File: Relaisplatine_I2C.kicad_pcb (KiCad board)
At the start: 2 copper layers, 85.1 x 107.3 mm, 35 parts, among them J1 J, J1.1 G1-J, J1.2 G1-K, J1001 Conn_01x08, J2 K, J2.1 G2-J, J2.2 G2-K, J3.1 G3-J, J3.2 G3-K, J4.1 G4-J, J4.2 G4-K, J5.1 G5-J, J5.2 G5-K, J6.1 G6-J, J6.2 G6-K, J7.1 G7-J, J7.2 G7-K, J8.1 G8-J, J8.2 G8-K, U1 ULN2803A, U2 PCF8574

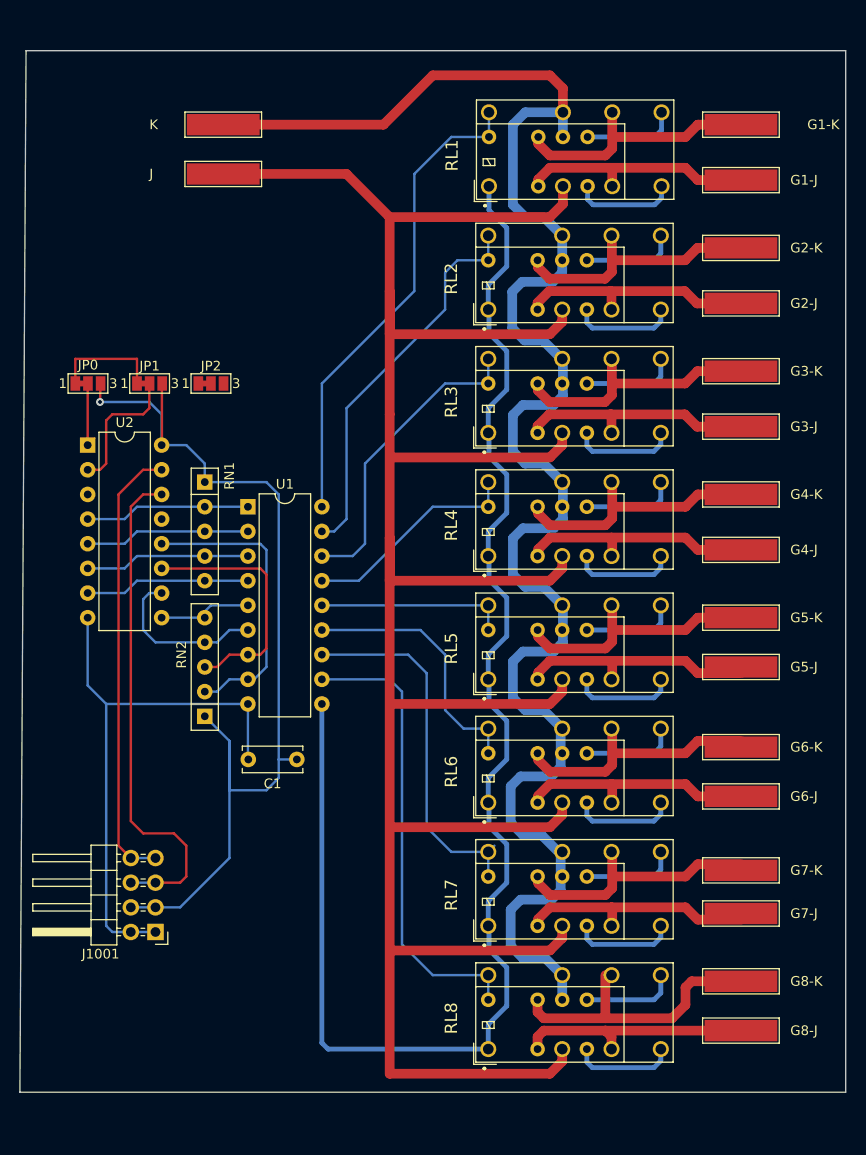
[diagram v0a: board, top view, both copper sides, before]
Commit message: Unbekannte Änderungen
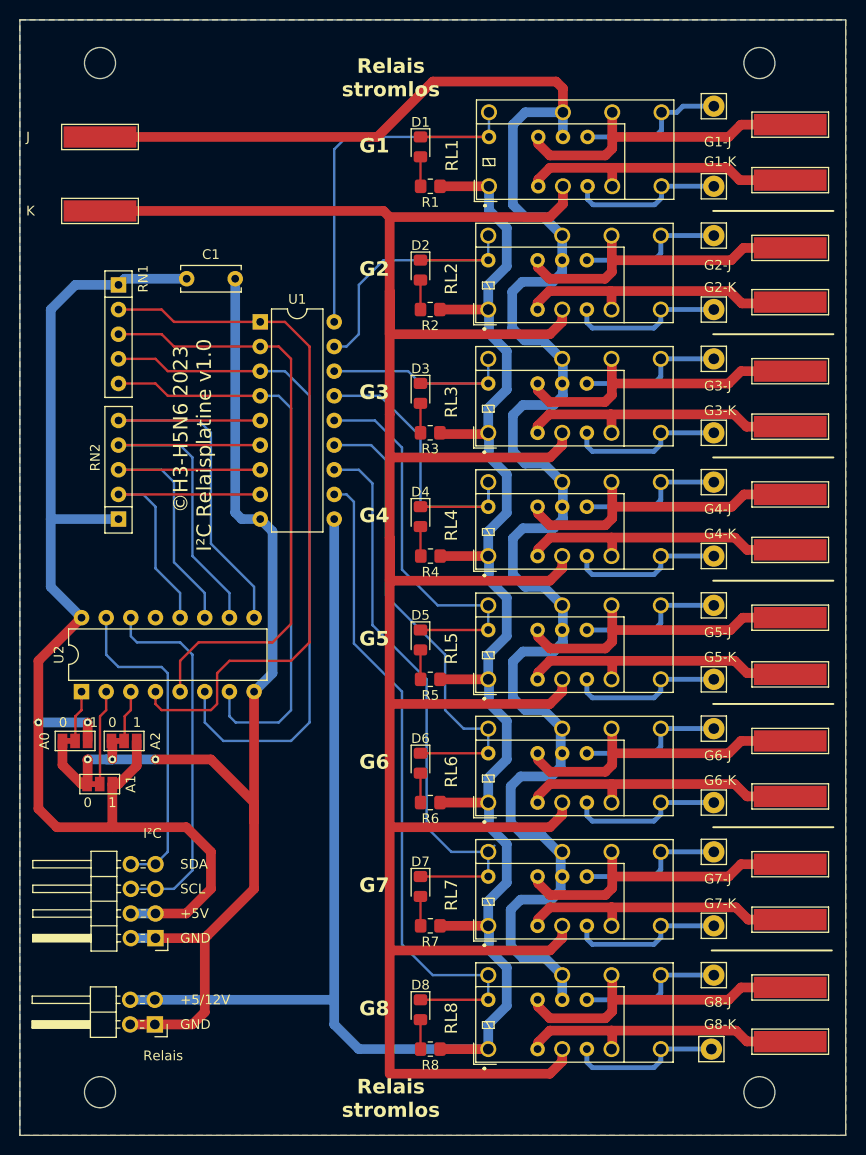
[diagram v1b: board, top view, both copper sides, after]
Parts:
- added D1: LED, LED_SMD:LED_0805_2012Metric_Pad1.15x1.40mm_HandSolder, F.Cu at (100.3, 56.9)
- added D2: LED, LED_SMD:LED_0805_2012Metric_Pad1.15x1.40mm_HandSolder, F.Cu at (100.3, 69.6)
- added D3: LED, LED_SMD:LED_0805_2012Metric_Pad1.15x1.40mm_HandSolder, F.Cu at (100.3, 82.3)
- added D4: LED, LED_SMD:LED_0805_2012Metric_Pad1.15x1.40mm_HandSolder, F.Cu at (100.3, 95.0)
- added D5: LED, LED_SMD:LED_0805_2012Metric_Pad1.15x1.40mm_HandSolder, F.Cu at (100.3, 107.7)
- added D6: LED, LED_SMD:LED_0805_2012Metric_Pad1.15x1.40mm_HandSolder, F.Cu at (100.3, 120.4)
- added D7: LED, LED_SMD:LED_0805_2012Metric_Pad1.15x1.40mm_HandSolder, F.Cu at (100.3, 133.1)
- added D8: LED, LED_SMD:LED_0805_2012Metric_Pad1.15x1.40mm_HandSolder, F.Cu at (100.3, 145.8)
- added H1: MountingHole, MountingHole:MountingHole_3.2mm_M3, F.Cu at (67.3, 48.3)
- added H2: MountingHole, MountingHole:MountingHole_3.2mm_M3, F.Cu at (67.3, 154.3)
- added H3: MountingHole, MountingHole:MountingHole_3.2mm_M3, F.Cu at (135.3, 48.3)
- added H4: MountingHole, MountingHole:MountingHole_3.2mm_M3, F.Cu at (135.3, 154.3)
- added J1.1a1001: G1-J, Connector_Pin:Pin_D1.1mm_L8.5mm_W2.5mm_FlatFork, F.Cu at (130.6, 52.7)
- added J1.1a1002: G1-K, Connector_Pin:Pin_D1.1mm_L8.5mm_W2.5mm_FlatFork, F.Cu at (130.6, 86.4)
- added J1.1a1003: G1-K, Connector_Pin:Pin_D1.1mm_L8.5mm_W2.5mm_FlatFork, F.Cu at (130.6, 99.1)
- added J1.1a1004: G1-K, Connector_Pin:Pin_D1.1mm_L8.5mm_W2.5mm_FlatFork, F.Cu at (130.6, 111.8)
- added J1.1a1005: G1-K, Connector_Pin:Pin_D1.1mm_L8.5mm_W2.5mm_FlatFork, F.Cu at (130.6, 124.5)
- added J1.1a1006: G1-K, Connector_Pin:Pin_D1.1mm_L8.5mm_W2.5mm_FlatFork, F.Cu at (130.6, 137.2)
- added J1.1a1007: G1-K, Connector_Pin:Pin_D1.1mm_L8.5mm_W2.5mm_FlatFork, F.Cu at (130.3, 149.9)
- added J1.2a1001: G1-K, Connector_Pin:Pin_D1.1mm_L8.5mm_W2.5mm_FlatFork, F.Cu at (130.6, 61.0)
- added J1.2a1002: G1-J, Connector_Pin:Pin_D1.1mm_L8.5mm_W2.5mm_FlatFork, F.Cu at (130.6, 78.7)
- added J1.2a1003: G1-J, Connector_Pin:Pin_D1.1mm_L8.5mm_W2.5mm_FlatFork, F.Cu at (130.6, 91.4)
- added J1.2a1004: G1-J, Connector_Pin:Pin_D1.1mm_L8.5mm_W2.5mm_FlatFork, F.Cu at (130.6, 104.1)
- added J1.2a1005: G1-J, Connector_Pin:Pin_D1.1mm_L8.5mm_W2.5mm_FlatFork, F.Cu at (130.6, 116.8)
- added J1.2a1006: G1-J, Connector_Pin:Pin_D1.1mm_L8.5mm_W2.5mm_FlatFork, F.Cu at (130.6, 129.5)
- added J1.2a1007: G1-J, Connector_Pin:Pin_D1.1mm_L8.5mm_W2.5mm_FlatFork, F.Cu at (130.6, 142.2)
- added J1001: I²C, Connector_PinHeader_2.54mm:PinHeader_2x02_P2.54mm_Horizontal, F.Cu at (73.0, 147.3)
- added J2.1a1001: G1-J, Connector_Pin:Pin_D1.1mm_L8.5mm_W2.5mm_FlatFork, F.Cu at (130.6, 66.0)
- added J2.2a1001: G2-K, Connector_Pin:Pin_D1.1mm_L8.5mm_W2.5mm_FlatFork, F.Cu at (130.6, 73.7)
- added R1: 1k, Resistor_SMD:R_0805_2012Metric_Pad1.20x1.40mm_HandSolder, F.Cu at (101.3, 61.0)
- added R2: 1k, Resistor_SMD:R_0805_2012Metric_Pad1.20x1.40mm_HandSolder, F.Cu at (101.3, 73.7)
- added R3: 1k, Resistor_SMD:R_0805_2012Metric_Pad1.20x1.40mm_HandSolder, F.Cu at (101.3, 86.4)
- added R4: 1k, Resistor_SMD:R_0805_2012Metric_Pad1.20x1.40mm_HandSolder, F.Cu at (101.4, 99.1)
- added R5: 1k, Resistor_SMD:R_0805_2012Metric_Pad1.20x1.40mm_HandSolder, F.Cu at (101.3, 111.8)
- added R6: 1k, Resistor_SMD:R_0805_2012Metric_Pad1.20x1.40mm_HandSolder, F.Cu at (101.3, 124.5)
- added R7: 1k, Resistor_SMD:R_0805_2012Metric_Pad1.20x1.40mm_HandSolder, F.Cu at (101.3, 137.2)
- added R8: 1k, Resistor_SMD:R_0805_2012Metric_Pad1.20x1.40mm_HandSolder, F.Cu at (101.3, 149.9)
- J1: value J -> K
- J1.1: value G1-J -> G1-K
- J1.2: value G1-K -> G1-J
- J10: renamed from J1001; value Conn_01x08 -> I²C
- J2: value K -> J
- J2.1: value G2-J -> G2-K
- J2.2: value G2-K -> G2-J
- J3.1: value G3-J -> G3-K
- J3.2: value G3-K -> G3-J
- J4.1: value G4-J -> G4-K
- J4.2: value G4-K -> G4-J
- J5.1: value G5-J -> G5-K
- J5.2: value G5-K -> G5-J
- J6.1: value G6-J -> G6-K
- J6.2: value G6-K -> G6-J
- J7.1: value G7-J -> G7-K
- J7.2: value G7-K -> G7-J
- J8.1: value G8-J -> G8-K
- J8.2: value G8-K -> G8-J
- moved C1 50.8 mm to (76.2, 70.5), turned to 0 degrees
- moved A1 41.6 mm to (67.3, 122.6)
- moved A2 37.9 mm to (69.8, 118.1)
- moved A0 36.9 mm to (64.7, 118.1)
- moved U2 25.4 mm to (65.4, 113.0), turned to 90 degrees
- moved RN1 22.2 mm to (69.2, 71.1)
- moved RN2 22.2 mm to (69.2, 95.2)
- moved U1 19.1 mm to (83.8, 74.9)
- moved J1 13.3 mm to (67.3, 63.5)
- moved J2 12.8 mm to (67.3, 55.9)
- moved J8.1 5.21 mm to (138.4, 149.1)
- moved J5.1 5.14 mm to (138.4, 111.3)
- moved J7.1 5.12 mm to (138.4, 136.5)
- moved J6.2 5.12 mm to (138.4, 118.1)
- moved J7.2 5.12 mm to (138.4, 130.8)
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- renumbered JP0 to A0, JP1 to A1, JP2 to A2
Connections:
- RL1 pad 5: unconnected-(RL1-Pad5) -> Net-(J1.2a1001-Pin_1)
- RL1 pad 8: unconnected-(RL1-Pad8) -> Net-(J1.1a1001-Pin_1)
- RL2 pad 5: unconnected-(RL2-Pad5) -> Net-(J2.2a1001-Pin_1)
- RL2 pad 8: unconnected-(RL2-Pad8) -> Net-(J2.1a1001-Pin_1)
- RL3 pad 5: unconnected-(RL3-Pad5) -> Net-(J1.1a1002-Pin_1)
- RL3 pad 8: unconnected-(RL3-Pad8) -> Net-(J1.2a1002-Pin_1)
- RL4 pad 5: unconnected-(RL4-Pad5) -> Net-(J1.1a1003-Pin_1)
- RL4 pad 8: unconnected-(RL4-Pad8) -> Net-(J1.2a1003-Pin_1)
- RL5 pad 5: unconnected-(RL5-Pad5) -> Net-(J1.1a1004-Pin_1)
- RL5 pad 8: unconnected-(RL5-Pad8) -> Net-(J1.2a1004-Pin_1)
- RL6 pad 5: unconnected-(RL6-Pad5) -> Net-(J1.1a1005-Pin_1)
- RL6 pad 8: unconnected-(RL6-Pad8) -> Net-(J1.2a1005-Pin_1)
- RL7 pad 5: unconnected-(RL7-Pad5) -> Net-(J1.1a1006-Pin_1)
- RL7 pad 8: unconnected-(RL7-Pad8) -> Net-(J1.2a1006-Pin_1)
- RL8 pad 5: unconnected-(RL8-Pad5) -> Net-(J1.1a1007-Pin_1)
- RL8 pad 8: unconnected-(RL8-Pad8) -> Net-(J1.2a1007-Pin_1)
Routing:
- net +12V: track 152.1 -> 229.7 mm
- net GND: track 69.7 -> 129.0 mm, vias 0 -> 3
- net Net-(RN1-R1): track 17.0 -> 73.9 mm
- net Net-(RN1-R3): track 17.0 -> 70.5 mm
- net Net-(RN1-R2): track 17.0 -> 62.3 mm
- net Net-(RN1-R4): track 17.0 -> 59.6 mm
- net Net-(RN2-R4): track 9.42 -> 45.5 mm
- net Net-(RN2-R3): track 17.2 -> 40.8 mm
- net +5V: track 103.4 -> 126.9 mm, vias 1 -> 2
- net Net-(D8-K): track 47.6 -> 69.7 mm
- net Net-(D7-K): track 38.3 -> 60.1 mm
- net Net-(D6-K): track 27.2 -> 49.0 mm
- net Net-(D5-K): track 19.8 -> 40.7 mm
- net Net-(J1.1a1004-Pin_1): track 0.00 -> 16.9 mm
- net Net-(J1.1a1002-Pin_1): track 0.00 -> 16.3 mm
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- added copper zone on F.Cu, net +5V
- added copper zone on B.Cu, net GND
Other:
- board size 85.1 x 107.3 mm -> 85.1 x 114.9 mm
- board text added: "+5/12V"
- board text added: "+5V"
- board text added: "G1"
- board text added: "G2"
- board text added: "G3"
- board text added: "G4"
- board text added: "G5"
- board text added: "G6"
- board text added: "G7"
- board text added: "G8"
- board text added: "GND"
- board text added: "Relais"
- board text added: "Relais stromlos"
- board text added: "SCL"
- board text added: "SDA"
- board text added: "©H3-H5N6 2023 I²C Relaisplatine v1.0"
